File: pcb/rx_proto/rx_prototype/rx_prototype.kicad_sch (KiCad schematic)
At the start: 53 parts, among them U1 nice_nano, U2 MPU-6500, U3 QMC5883P, U4 MCP6004, U5 MCP6004, U6 74HC4051

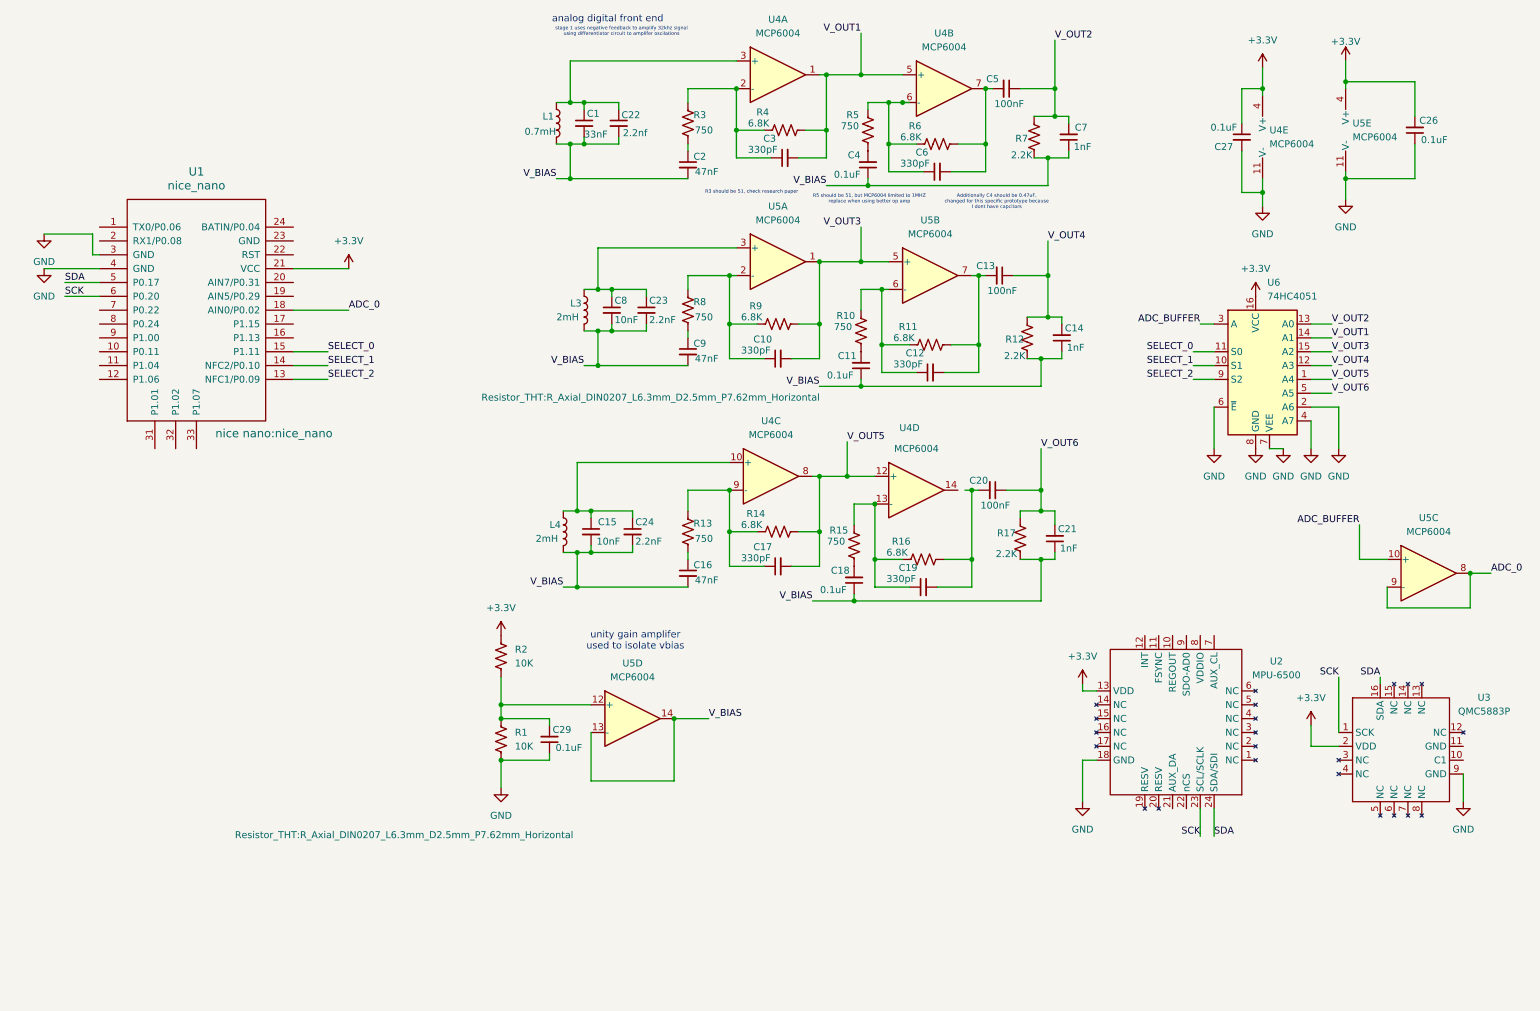
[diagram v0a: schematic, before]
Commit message: Update perf layout
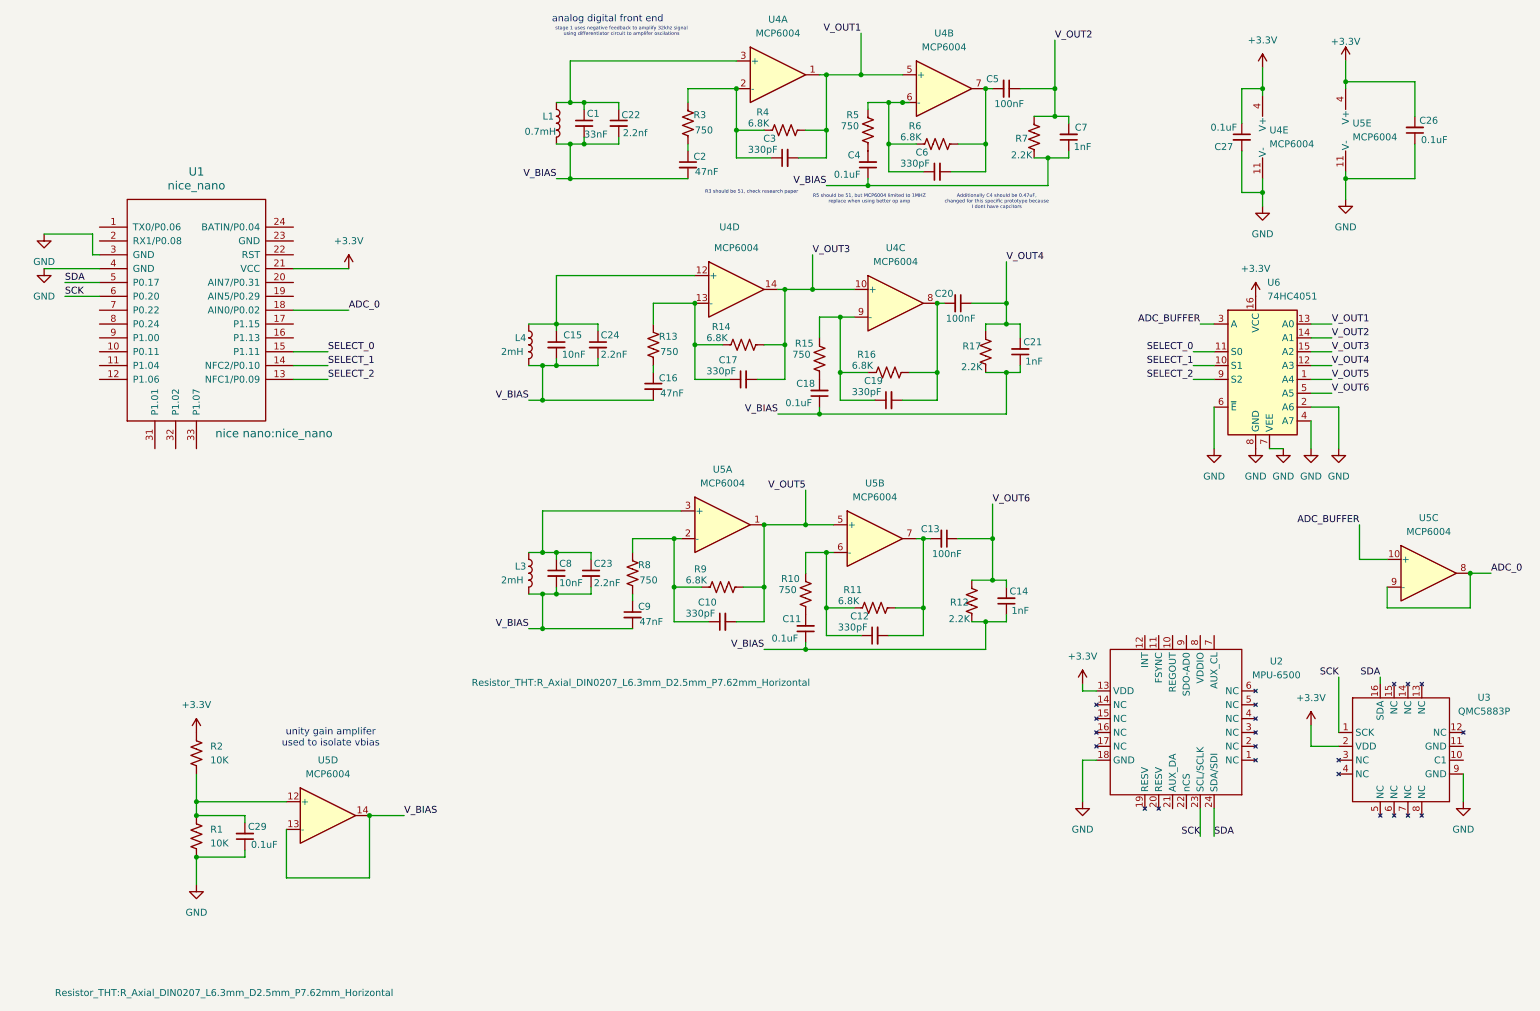
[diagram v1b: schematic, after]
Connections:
- net V_OUT1: now also U6.13 (A0); no longer U6.14 (A1)
- net V_OUT2: now also U6.14 (A1); no longer U6.13 (A0)
- net V_OUT3: now also C17.2, R14.1, U4.10 (+), U4.14; no longer C10.2, R9.1, U5.1, U5.5 (+)
- net V_OUT4: now also C20.1, C21.2, R17.1; no longer C13.1, C14.2, R12.1
- net V_OUT5: now also C10.2, R9.1, U5.1, U5.5 (+); no longer C17.2, R14.1, U4.12 (+), U4.8
- net V_OUT6: now also C13.1, C14.2, R12.1; no longer C20.1, C21.2, R17.1
- net at C19.1, R15.1, R16.2: now also U4.9 (-); no longer U4.13 (-)
- net at C15.1, C24.1, L4.1: now also U4.12 (+); no longer U4.10 (+)
- net at C17.1, R13.1, R14.2: now also U4.13 (-); no longer U4.9 (-)
- net at C19.2, C20.2, R16.1: now also U4.8
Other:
- moved on the sheet: C10, C11, C12, C13, C14, C15, C16, C17, C18, C19, C20, C21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
